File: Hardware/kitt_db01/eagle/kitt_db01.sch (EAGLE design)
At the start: 40 parts, among them Q1 [MMBF170], U1 ADNS-3080, U2 MIC5205-3.3YM5TR, X1 RESON

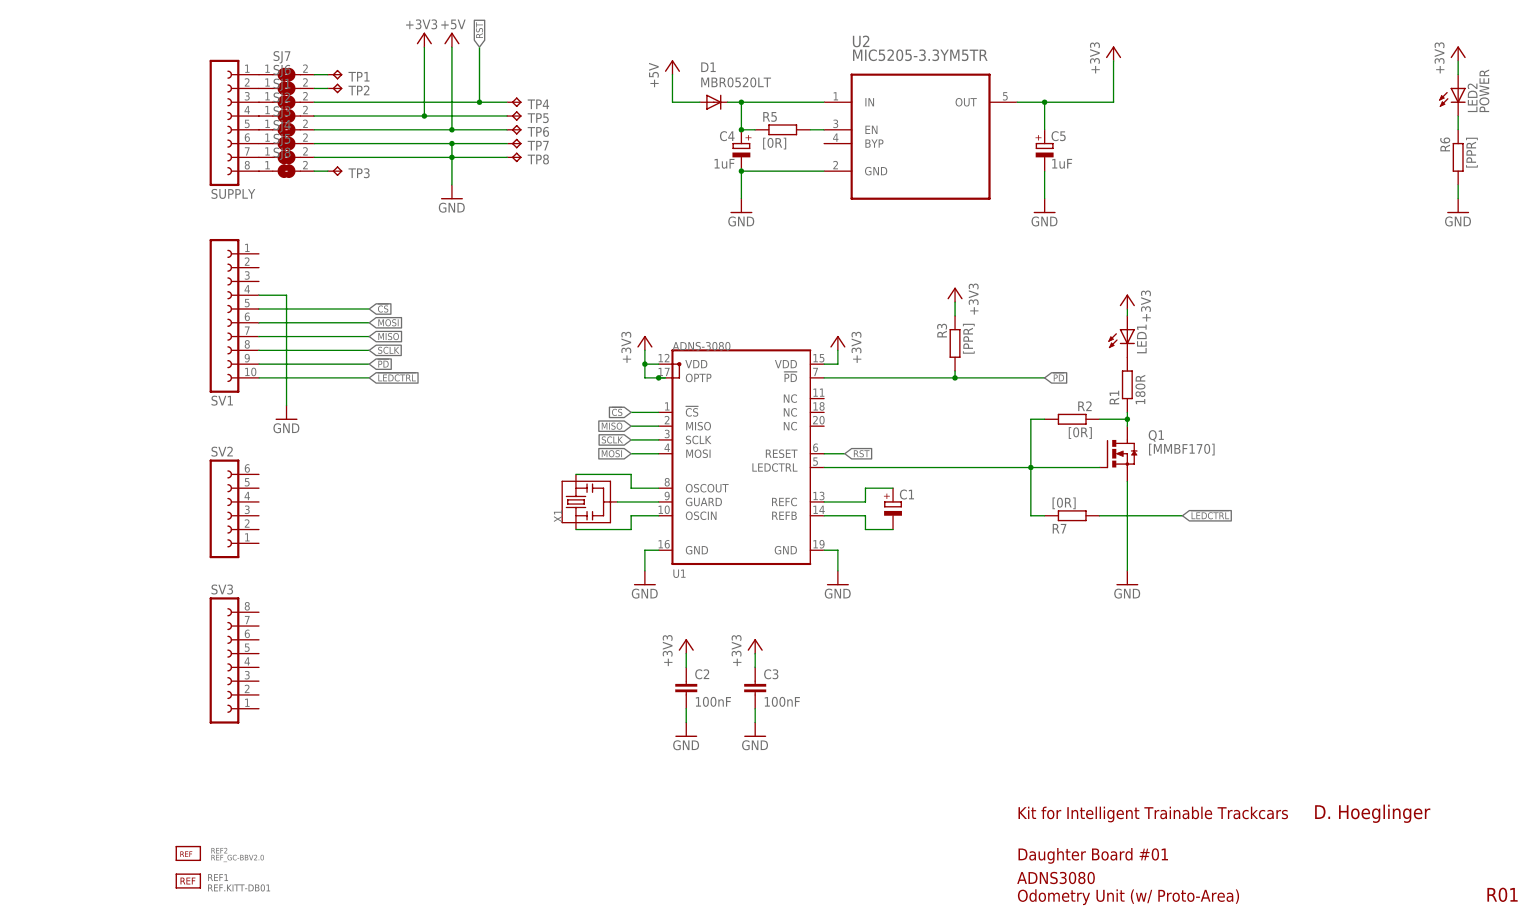
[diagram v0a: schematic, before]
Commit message: snapshot of board db01 + added southwest patching area
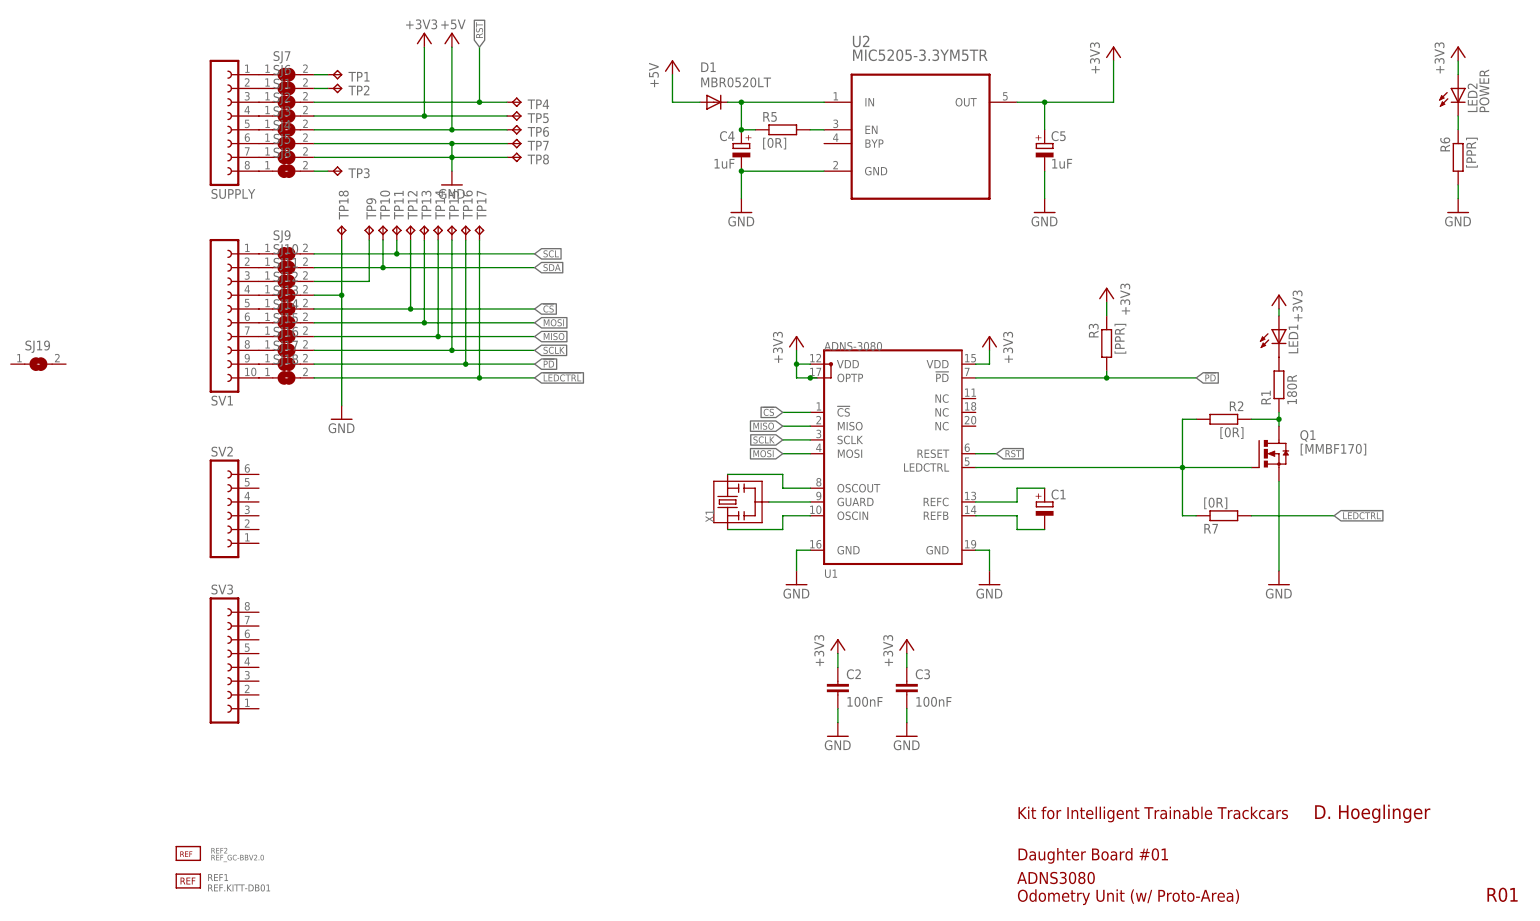
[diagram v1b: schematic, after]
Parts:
- added SJ10, SJ11, SJ12, SJ13, SJ14, SJ15, SJ16, SJ17, SJ18, SJ19, SJ9: (no value), jumper:SJ
- added TP10, TP11, TP12, TP13, TP14, TP15, TP16, TP17, TP18, TP9: TPPAD1-13, testpad:TPPAD1-13
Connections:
- new net N$143: SJ9.1, SV1.1
- new net N$144: SJ10.1, SV1.2
- new net N$145: SJ11.1, SV1.3
- new net N$146: SJ11.2, TP9.TP
- new net N$147: SJ12.1, SV1.4
- new net N$148: SJ13.1, SV1.5
- new net N$149: SJ14.1, SV1.6
- new net N$150: SJ15.1, SV1.7
- new net N$151: SJ16.1, SV1.8
- new net N$152: SJ17.1, SV1.9
- new net N$153: SJ18.1, SV1.10
- new net SCL: SJ9.2, TP11.TP
- new net SDA: SJ10.2, TP10.TP
- net !CS: now also SJ13.2, TP12.TP; no longer SV1.5
- net !LEDCTRL: now also SJ18.2, TP17.TP; no longer SV1.10
- net !PD: now also SJ17.2, TP16.TP; no longer SV1.9
- net GND: now also SJ12.2, TP18.TP; no longer SV1.4
- net MISO: now also SJ15.2, TP14.TP; no longer SV1.7
- net MOSI: now also SJ14.2, TP13.TP; no longer SV1.6
- net SCLK: now also SJ16.2, TP15.TP; no longer SV1.8
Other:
- moved on the sheet: C1, C2, C3, LED1, Q1, R1, R2, R3, R7, U1, X1
